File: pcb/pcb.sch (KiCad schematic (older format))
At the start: 17 parts, among them J1 Barrel_Jack, J2 Barrel_Jack, J3 Screw_Terminal_01x03, J4 Screw_Terminal_01x02, J5 Conn_02x05_Odd_Even, J6 Conn_01x06_Male, SW1 SW_SPDT, U1 CPC5001G

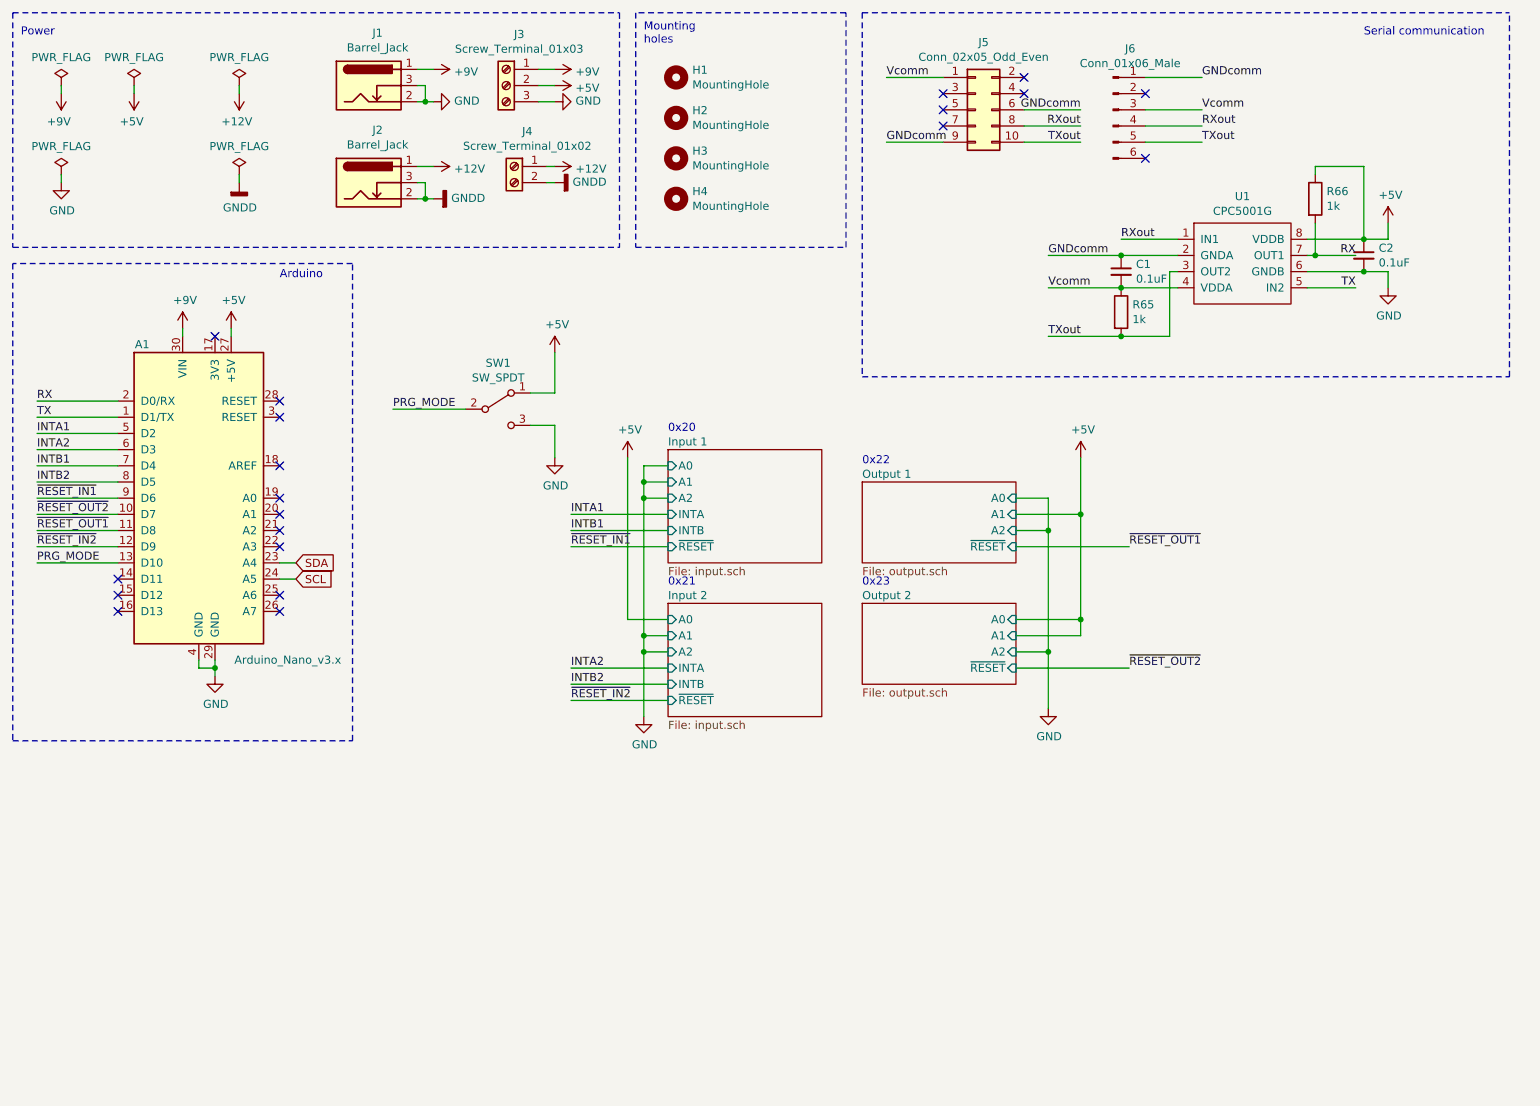
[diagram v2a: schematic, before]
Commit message: latest
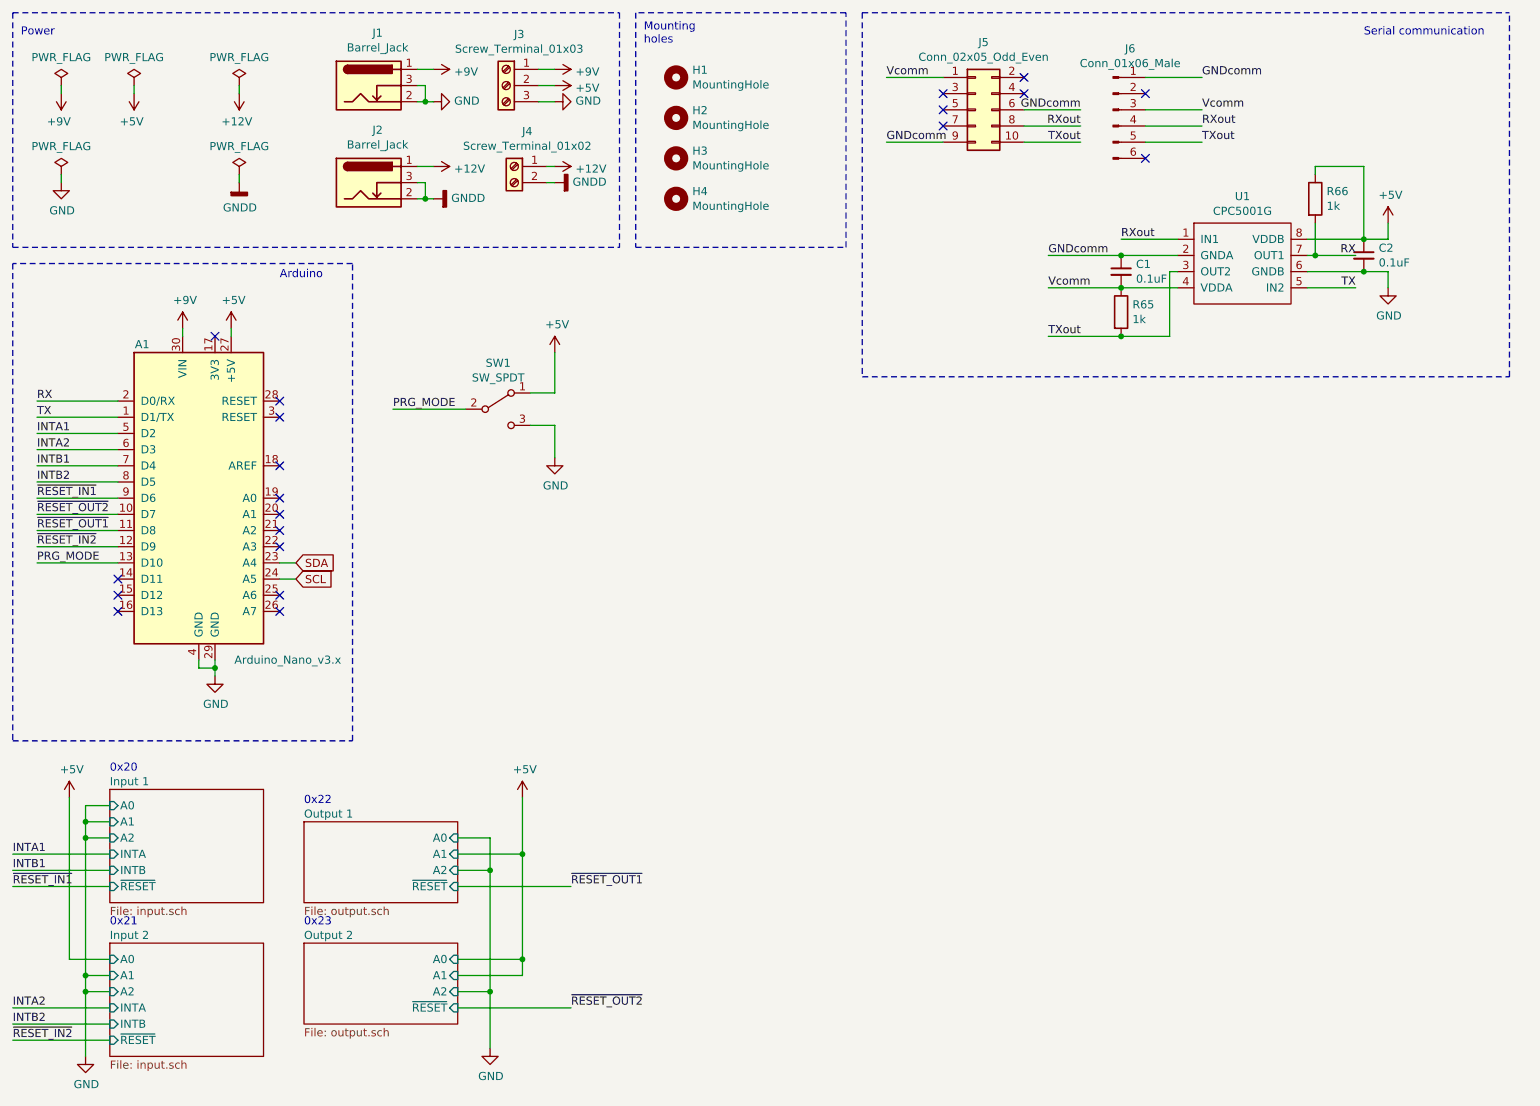
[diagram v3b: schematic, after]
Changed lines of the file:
@@
 Power
 $Sheet
-S 4850 3550 950  700
+S 1400 5650 950  700
 U 5C211542
 F0 "Input 1" 50
 F1 "input.sch" 50
-F2 "A0" I L 4850 3650 50
-F3 "A1" I L 4850 3750 50
-F4 "A2" I L 4850 3850 50
-F5 "INTA" I L 4850 3950 50
-F6 "INTB" I L 4850 4050 50
-F7 "~RESET" I L 4850 4150 50
+F2 "A0" I L 1400 5750 50
+F3 "A1" I L 1400 5850 50
+F4 "A2" I L 1400 5950 50
+F5 "INTA" I L 1400 6050 50
+F6 "INTB" I L 1400 6150 50
+F7 "~RESET" I L 1400 6250 50
 $EndSheet
 $Sheet
-S 4850 4500 950  700
+S 1400 6600 950  700
 U 5C211551
 F0 "Input 2" 50
 F1 "input.sch" 50
-F2 "A0" I L 4850 4600 50
-F3 "A1" I L 4850 4700 50
-F4 "A2" I L 4850 4800 50
-F5 "INTA" I L 4850 4900 50
-F6 "INTB" I L 4850 5000 50
-F7 "~RESET" I L 4850 5100 50
+F2 "A0" I L 1400 6700 50
+F3 "A1" I L 1400 6800 50
+F4 "A2" I L 1400 6900 50
+F5 "INTA" I L 1400 7000 50
+F6 "INTB" I L 1400 7100 50
+F7 "~RESET" I L 1400 7200 50
 $EndSheet
 $Comp
 L power:GND #PWR019
 U 1 1 5C24134C
-P 4700 5200
-F 0 "#PWR019" H 4700 4950 50  0001 C CNN
-F 1 "GND" H 4705 5027 50  0000 C CNN
-F 2 "" H 4700 5200 50  0001 C CNN
-F 3 "" H 4700 5200 50  0001 C CNN
-	1    4700 5200
+P 1250 7300
+F 0 "#PWR019" H 1250 7050 50  0001 C CNN
+F 1 "GND" H 1255 7127 50  0000 C CNN
+F 2 "" H 1250 7300 50  0001 C CNN
+F 3 "" H 1250 7300 50  0001 C CNN
+	1    1250 7300
 	1    0    0    -1
 $EndComp
@@
 L power:+5V #PWR018
 U 1 1 5C2413B9
-P 4600 3600
-F 0 "#PWR018" H 4600 3450 50  0001 C CNN
-F 1 "+5V" H 4615 3773 50  0000 C CNN
-F 2 "" H 4600 3600 50  0001 C CNN
-F 3 "" H 4600 3600 50  0001 C CNN
-	1    4600 3600
-	1    0    0    -1
-$EndComp
-Wire Wire Line
-	4850 3650 4700 3650
-Wire Wire Line
-	4700 3650 4700 3750
-Wire Wire Line
-	4850 3750 4700 3750
-Connection ~ 4700 3750
-Wire Wire Line
-	4700 3750 4700 3850
-Wire Wire Line
-	4850 3850 4700 3850
-Wire Wire Line
-	4850 4700 4700 4700
-Wire Wire Line
-	4700 4700 4700 4800
-Wire Wire Line
-	4850 4800 4700 4800
-Text Notes 4850 3450 0    50   ~ 0
+P 1150 5700
+F 0 "#PWR018" H 1150 5550 50  0001 C CNN
+F 1 "+5V" H 1165 5873 50  0000 C CNN
+F 2 "" H 1150 5700 50  0001 C CNN
+F 3 "" H 1150 5700 50  0001 C CNN
+	1    1150 5700
+	1    0    0    -1
+$EndComp
+Wire Wire Line
+	1400 5750 1250 5750
+Wire Wire Line
+	1250 5750 1250 5850
+Wire Wire Line
+	1400 5850 1250 5850
+Connection ~ 1250 5850
+Wire Wire Line
+	1250 5850 1250 5950
+Wire Wire Line
+	1400 5950 1250 5950
+Wire Wire Line
+	1400 6800 1250 6800
+Wire Wire Line
+	1250 6800 1250 6900
+Wire Wire Line
+	1400 6900 1250 6900
+Text Notes 1400 5550 0    50   ~ 0
 0x20
-Text Notes 4850 4400 0    50   ~ 0
+Text Notes 1400 6500 0    50   ~ 0
 0x21
 $Sheet
-S 6050 3750 950  500
+S 2600 5850 950  500
 U 5C242719
 F0 "Output 1" 50
 F1 "output.sch" 50
-F2 "A0" I R 7000 3850 50
-F3 "A1" I R 7000 3950 50
-F4 "A2" I R 7000 4050 50
-F5 "~RESET" I R 7000 4150 50
+F2 "A0" I R 3550 5950 50
+F3 "A1" I R 3550 6050 50
+F4 "A2" I R 3550 6150 50
+F5 "~RESET" I R 3550 6250 50
 $EndSheet
 $Sheet
-S 6050 4500 950  500
+S 2600 6600 950  500
 U 5C24272E
 F0 "Output 2" 50
 F1 "output.sch" 50
-F2 "A0" I R 7000 4600 50
-F3 "A1" I R 7000 4700 50
-F4 "A2" I R 7000 4800 50
-F5 "~RESET" I R 7000 4900 50
+F2 "A0" I R 3550 6700 50
+F3 "A1" I R 3550 6800 50
+F4 "A2" I R 3550 6900 50
+F5 "~RESET" I R 3550 7000 50
 $EndSheet
 $Comp
 L power:GND #PWR020
 U 1 1 5C2430F8
-P 7200 5150
-F 0 "#PWR020" H 7200 4900 50  0001 C CNN
-F 1 "GND" H 7205 4977 50  0000 C CNN
-F 2 "" H 7200 5150 50  0001 C CNN
-F 3 "" H 7200 5150 50  0001 C CNN
-	1    7200 5150
-	1    0    0    -1
-$EndComp
-Wire Wire Line
-	7000 4050 7200 4050
-Wire Wire Line
-	7200 4050 7200 4800
-Wire Wire Line
-	7000 4800 7200 4800
-Connection ~ 7200 4800
-Wire Wire Line
-	7200 4800 7200 5150
-Wire Wire Line
-	7000 3850 7200 3850
-Wire Wire Line
-	7200 3850 7200 4050
-Connection ~ 7200 4050
+P 3750 7250
+F 0 "#PWR020" H 3750 7000 50  0001 C CNN
+F 1 "GND" H 3755 7077 50  0000 C CNN
+F 2 "" H 3750 7250 50  0001 C CNN
+F 3 "" H 3750 7250 50  0001 C CNN
+	1    3750 7250
+	1    0    0    -1
+$EndComp
+Wire Wire Line
+	3550 6150 3750 6150
+Wire Wire Line
+	3750 6150 3750 6900
+Wire Wire Line
+	3550 6900 3750 6900
+Connection ~ 3750 6900
+Wire Wire Line
+	3750 6900 3750 7250
+Wire Wire Line
+	3550 5950 3750 5950
+Wire Wire Line
+	3750 5950 3750 6150
+Connection ~ 3750 6150
 $Comp
 L power:+5V #PWR021
 U 1 1 5C243E0C
-P 7400 3600
-F 0 "#PWR021" H 7400 3450 50  0001 C CNN
-F 1 "+5V" H 7415 3773 50  0000 C CNN
-F 2 "" H 7400 3600 50  0001 C CNN
-F 3 "" H 7400 3600 50  0001 C CNN
-	1    7400 3600
-	1    0    0    -1
-$EndComp
-Wire Wire Line
-	7400 3600 7400 3950
-Wire Wire Line
-	7400 3950 7000 3950
-Wire Wire Line
-	7400 3950 7400 4600
-Wire Wire Line
-	7400 4600 7000 4600
-Connection ~ 7400 3950
-Wire Wire Line
-	7000 4700 7400 4700
-Wire Wire Line
-	7400 4700 7400 4600
-Connection ~ 7400 4600
+P 3950 5700
+F 0 "#PWR021" H 3950 5550 50  0001 C CNN
+F 1 "+5V" H 3965 5873 50  0000 C CNN
+F 2 "" H 3950 5700 50  0001 C CNN
+F 3 "" H 3950 5700 50  0001 C CNN
+	1    3950 5700
+	1    0    0    -1
+$EndComp
+Wire Wire Line
+	3950 5700 3950 6050
+Wire Wire Line
+	3950 6050 3550 6050
+Wire Wire Line
+	3950 6050 3950 6700
+Wire Wire Line
+	3950 6700 3550 6700
+Connection ~ 3950 6050
+Wire Wire Line
+	3550 6800 3950 6800
+Wire Wire Line
+	3950 6800 3950 6700
+Connection ~ 3950 6700
 $Comp
 L Connector:Screw_Terminal_01x02 J4
@@
 $EndComp
 Wire Wire Line
-	4600 3600 4600 4600
-Wire Wire Line
-	4250 3950 4850 3950
-Wire Wire Line
-	4250 4050 4850 4050
-Wire Wire Line
-	4250 5000 4850 5000
-Text Label 4250 3950 0    50   ~ 0
+	1150 5700 1150 6700
+Wire Wire Line
+	800  6050 1400 6050
+Wire Wire Line
+	800  6150 1400 6150
+Wire Wire Line
+	800  7100 1400 7100
+Text Label 800  6050 0    50   ~ 0
 INTA1
-Text Label 4250 4050 0    50   ~ 0
+Text Label 800  6150 0    50   ~ 0
 INTB1
-Text Label 4250 4900 0    50   ~ 0
+Text Label 800  7000 0    50   ~ 0
 INTA2
-Text Label 4250 5000 0    50   ~ 0
+Text Label 800  7100 0    50   ~ 0
 INTB2
 Text Label 950  3450 0    50   ~ 0
@@
 INTB2
 Wire Wire Line
-	4250 4150 4850 4150
-Text Label 4250 4150 0    50   ~ 0
+	800  6250 1400 6250
+Text Label 800  6250 0    50   ~ 0
 ~RESET_IN1
 Wire Wire Line
-	4250 4900 4850 4900
-Wire Wire Line
-	4700 5200 4700 4800
-Connection ~ 4700 4800
-Wire Wire Line
-	4600 4600 4850 4600
-Wire Wire Line
-	4700 3850 4700 4700
-Connection ~ 4700 3850
-Connection ~ 4700 4700
-Wire Wire Line
-	4850 5100 4250 5100
-Text Label 4250 5100 0    50   ~ 0
+	800  7000 1400 7000
+Wire Wire Line
+	1250 7300 1250 6900
+Connection ~ 1250 6900
+Wire Wire Line
+	1150 6700 1400 6700
+Wire Wire Line
+	1250 5950 1250 6800
+Connection ~ 1250 5950
+Connection ~ 1250 6800
+Wire Wire Line
+	1400 7200 800  7200
+Text Label 800  7200 0    50   ~ 0
 ~RESET_IN2
 Wire Wire Line
-	7000 4150 7700 4150
-Wire Wire Line
-	7000 4900 7700 4900
-Text Label 7700 4150 0    50   ~ 0
+	3550 6250 4250 6250
+Wire Wire Line
+	3550 7000 4250 7000
+Text Label 4250 6250 0    50   ~ 0
 ~RESET_OUT1
-Text Label 7700 4900 0    50   ~ 0
+Text Label 4250 7000 0    50   ~ 0
 ~RESET_OUT2
 Text Label 950  3850 0    50   ~ 0
@@
 Text Label 8150 1550 0    50   ~ 0
 RXout
-Text Notes 6050 3650 0    50   ~ 0
+Text Notes 2600 5750 0    50   ~ 0
 0x22
-Text Notes 6050 4400 0    50   ~ 0
+Text Notes 2600 6500 0    50   ~ 0
 0x23
 Wire Notes Line
@@
 NoConn ~ 7800 1750
 Wire Notes Line
-	6050 850  6050 3100
-Wire Notes Line
-	10050 3100 10050 850
-Wire Notes Line
 	6050 850  10050 850
-Wire Notes Line
-	6050 3100 10050 3100
 $Comp
 L pcb:CPC5001G U1
@@
 Wire Wire Line
 	9150 2450 9300 2450
+Wire Notes Line
+	6050 850  6050 3100
+Wire Notes Line
+	6050 3100 10050 3100
+Wire Notes Line
+	10050 3100 10050 850
 $EndSCHEMATC
